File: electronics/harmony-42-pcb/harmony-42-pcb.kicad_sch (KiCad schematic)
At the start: 12 parts

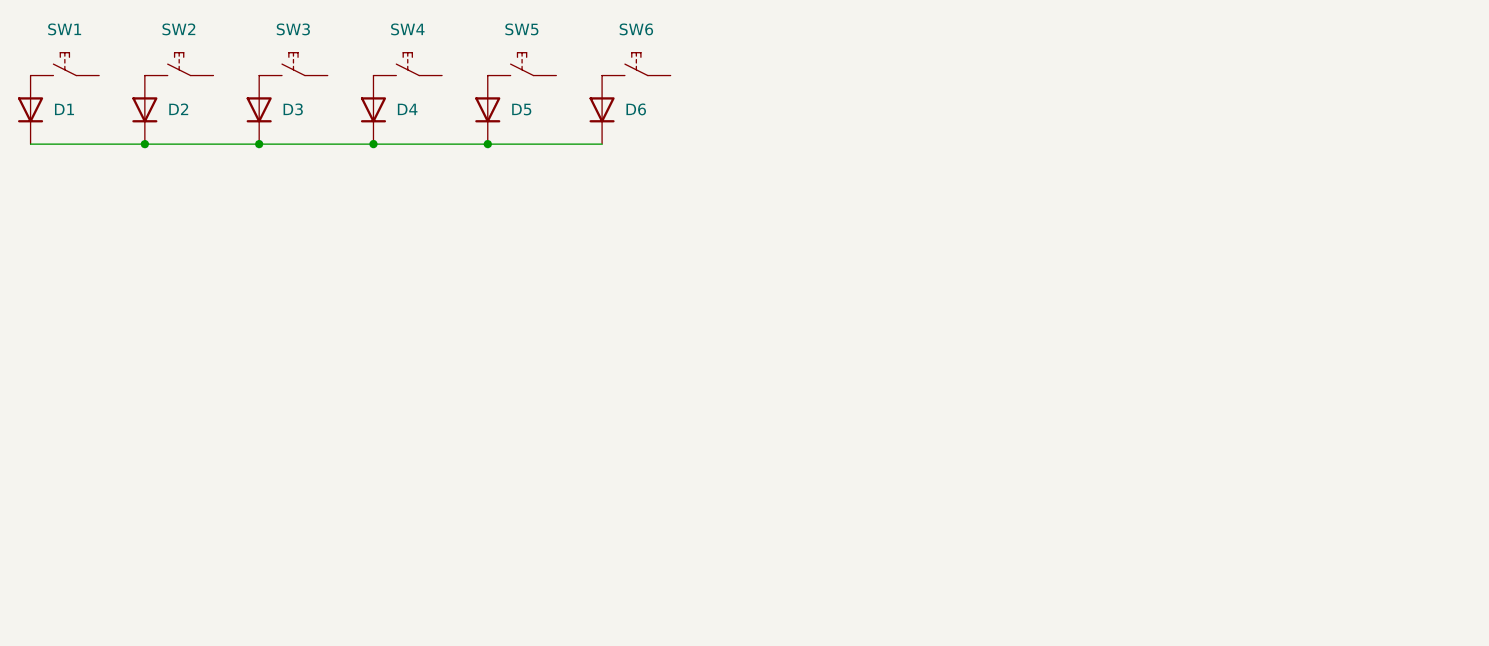
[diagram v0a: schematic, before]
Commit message: Add keys
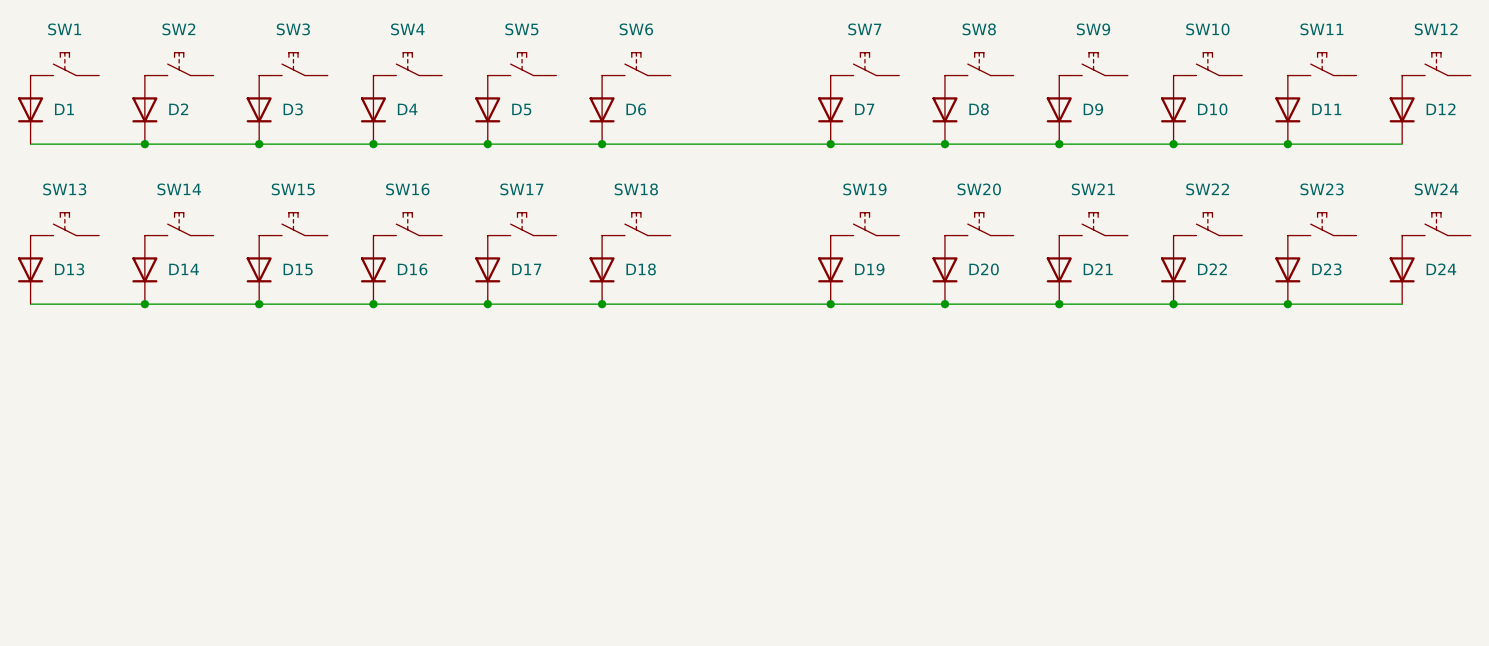
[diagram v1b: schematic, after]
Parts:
- added D10, D11, D12, D13, D14, D15, D16, D17, D18, D19, D20, D21, D22, D23, D24, D7, D8, D9: 1N4148WS, Project_Library:D_SOD-323F, symbol Diode:1N4148WS
- added SW10, SW11, SW12, SW13, SW14, SW15, SW16, SW17, SW18, SW19, SW20, SW21, SW22, SW23, SW24, SW7, SW8, SW9: ~, Project_Library:Hot_Swap_Socket_CPG151101S11, symbol Project_Library:SW_Hot_Swap_Socket
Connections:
- net at D1.1 (K), D2.1 (K), D3.1 (K)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: now also D10.1 (K), D11.1 (K), D12.1 (K), D7.1 (K), D8.1 (K), D9.1 (K)
- new net: D13.1 (K), D14.1 (K), D15.1 (K), D16.1 (K), D17.1 (K), D18.1 (K), D19.1 (K), D20.1 (K), D21.1 (K), D22.1 (K), D23.1 (K), D24.1 (K)
- new net: D24.2 (A), SW24.2
- new net: D22.2 (A), SW22.2
- new net: D23.2 (A), SW23.2
- new net: D21.2 (A), SW21.2
- new net: D12.2 (A), SW12.2
- new net: D11.2 (A), SW11.2
- new net: D20.2 (A), SW20.2
- new net: D8.2 (A), SW8.2
- new net: D15.2 (A), SW15.2
- new net: D7.2 (A), SW7.2
- new net: D13.2 (A), SW13.2
- new net: D19.2 (A), SW19.2
- new net: D10.2 (A), SW10.2
- new net: D9.2 (A), SW9.2
- new net: D16.2 (A), SW16.2
- new net: D14.2 (A), SW14.2
- new net: D17.2 (A), SW17.2
- new net: D18.2 (A), SW18.2

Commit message: Add keys
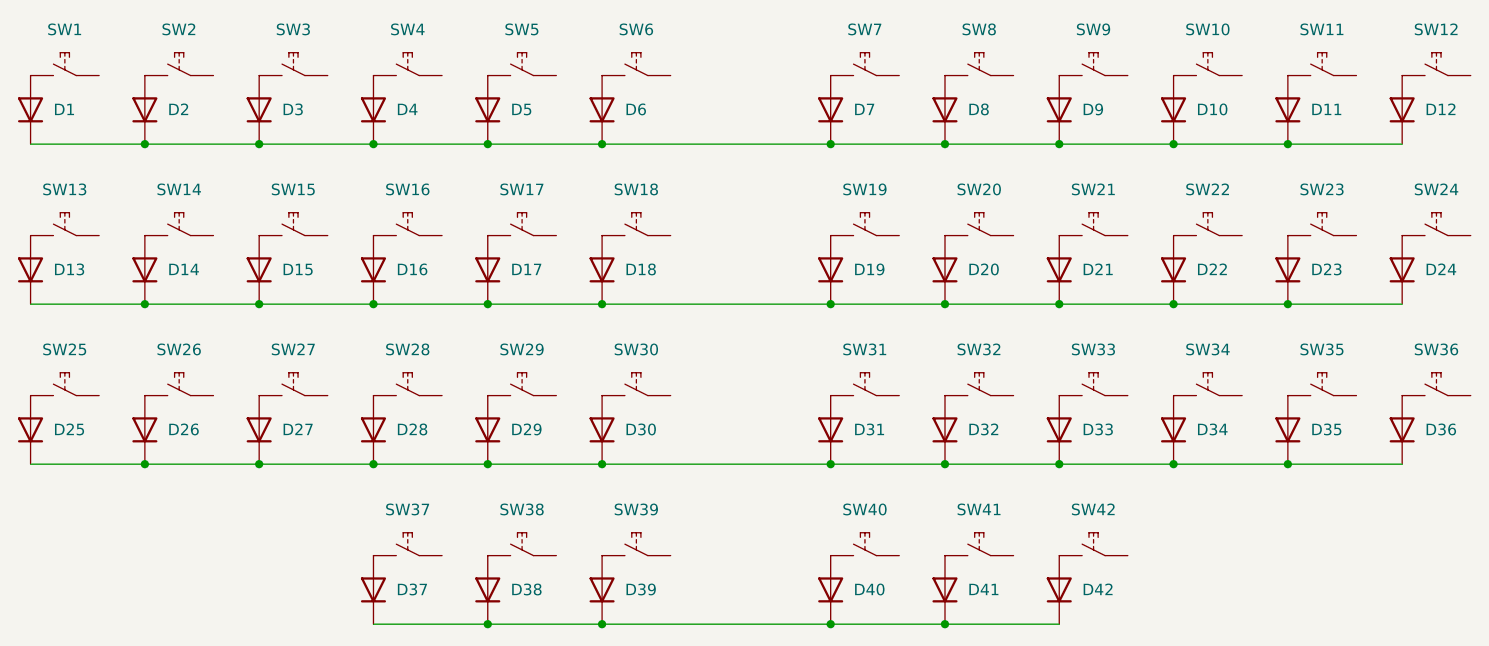
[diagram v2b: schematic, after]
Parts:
- added D25, D26, D27, D28, D29, D30, D31, D32, D33, D34, D35, D36, D37, D38, D39, D40, D41, D42: 1N4148WS, Project_Library:D_SOD-323F, symbol Diode:1N4148WS
- added SW25, SW26, SW27, SW28, SW29, SW30, SW31, SW32, SW33, SW34, SW35, SW36, SW37, SW38, SW39, SW40, SW41, SW42: ~, Project_Library:Hot_Swap_Socket_CPG151101S11, symbol Project_Library:SW_Hot_Swap_Socket
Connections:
- new net: D25.1 (K), D26.1 (K), D27.1 (K), D28.1 (K), D29.1 (K), D30.1 (K), D31.1 (K), D32.1 (K), D33.1 (K), D34.1 (K), D35.1 (K), D36.1 (K)
- new net: D31.2 (A), SW31.2
- new net: D34.2 (A), SW34.2
- new net: D38.2 (A), SW38.2
- new net: D27.2 (A), SW27.2
- new net: D28.2 (A), SW28.2
- new net: D37.1 (K), D38.1 (K), D39.1 (K), D40.1 (K), D41.1 (K), D42.1 (K)
- new net: D40.2 (A), SW40.2
- new net: D41.2 (A), SW41.2
- new net: D33.2 (A), SW33.2
- new net: D42.2 (A), SW42.2
- new net: D29.2 (A), SW29.2
- new net: D30.2 (A), SW30.2
- new net: D32.2 (A), SW32.2
- new net: D36.2 (A), SW36.2
- new net: D39.2 (A), SW39.2
- new net: D26.2 (A), SW26.2
- new net: D37.2 (A), SW37.2
- new net: D25.2 (A), SW25.2
- new net: D35.2 (A), SW35.2
